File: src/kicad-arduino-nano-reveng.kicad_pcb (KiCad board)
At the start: 2 copper layers, 43.8 x 18.4 mm, 29 parts, among them J1 USB_B_Mini, J2 ISP, J3 Conn_01x15, J4 Conn_01x15, SW1 RESET, U1 AMS1117-5.0, U2 ATmega328P-AU, U3 CH340G, Y1 Crystal_Atmega, Y2 Crystal

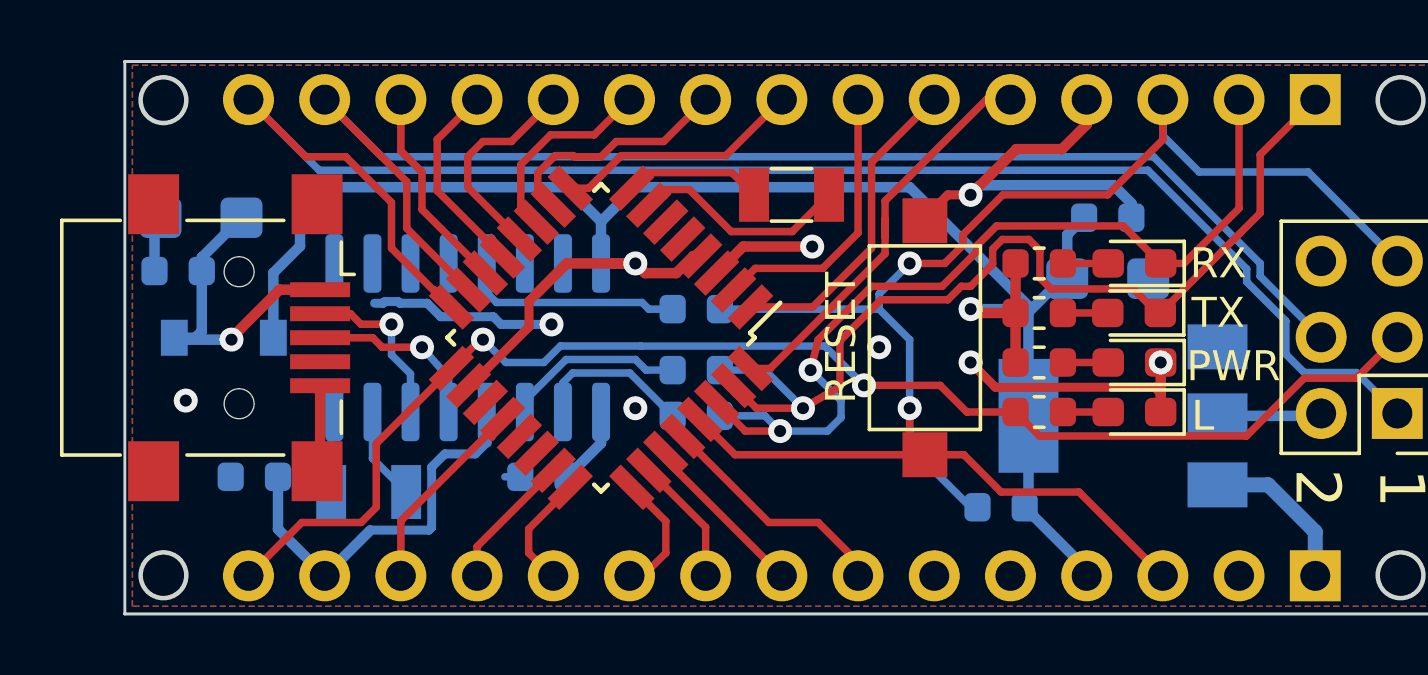
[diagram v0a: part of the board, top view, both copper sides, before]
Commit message: Finished wiring
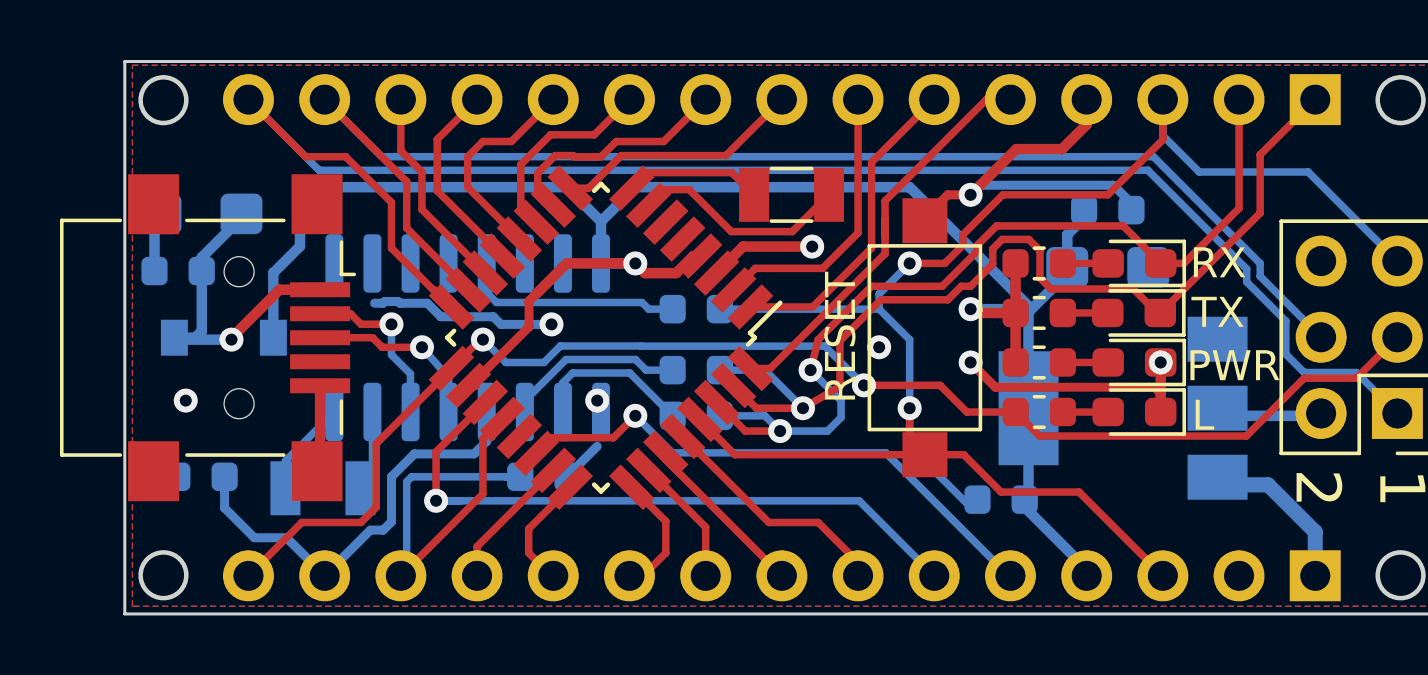
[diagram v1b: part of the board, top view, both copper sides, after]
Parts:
- U1: footprint Package_TO_SOT_SMD:SOT-223-3_TabPin2 -> igorkelvin:SOT-223-3_TabPin2
- moved C5 1.78 mm to (80.0, 61.5)
- moved Y2 1.53 mm to (84.1, 61.8)
- moved C1 0.38 mm to (110.2, 54.5)
- moved R1 0.25 mm to (106.7, 62.2)
- moved C2 0.25 mm to (110.2, 52.6)
- moved U1 0.25 mm to (110.7, 59.2)
- moved C6 0.13 mm to (80.0, 52.7)
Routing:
- net A6: track 0.00 -> 22.4 mm, vias 0 -> 1
- net A7: track 0.00 -> 18.5 mm
- net AREF: track 7.30 -> 14.4 mm
- net 3V3: track 13.4 -> 15.4 mm
- net GND: track 40.3 -> 39.3 mm, vias 7 -> 8
- net XO: track 2.71 -> 3.34 mm

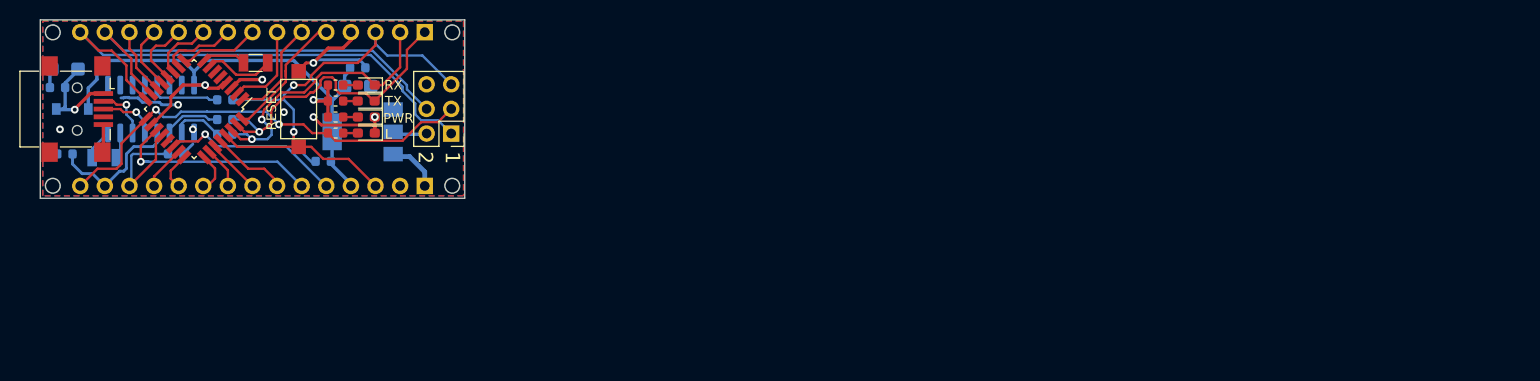
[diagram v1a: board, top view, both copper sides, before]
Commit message: PCB Rev0
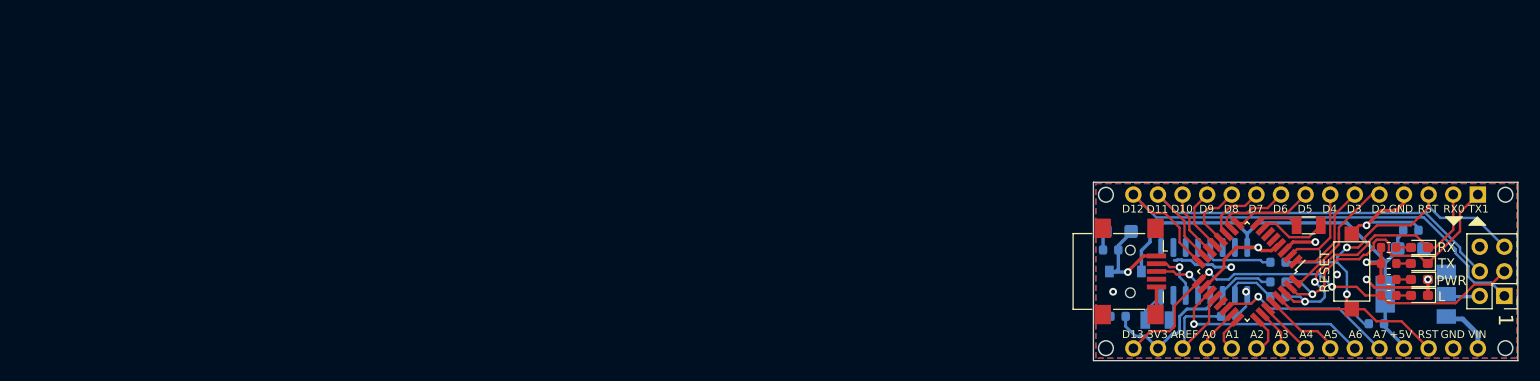
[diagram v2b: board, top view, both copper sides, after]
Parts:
- moved Y1 110.0 mm to (208.4, 68.8)
- moved C1 110.0 mm to (218.9, 71.2)
- moved C2 110.0 mm to (218.9, 69.3)
- moved C3 110.0 mm to (205.2, 72.6)
- moved C5 110.0 mm to (188.7, 78.2)
- moved C6 110.0 mm to (188.7, 69.5)
- moved C7 110.0 mm to (188.0, 71.4)
- moved D2 110.0 mm to (219.8, 72.8)
- moved D5 110.0 mm to (189.5, 73.6)
- moved R2 110.0 mm to (205.2, 74.7)
- moved R3 110.0 mm to (205.2, 76.2)
- moved R4 110.0 mm to (216.7, 71.1)
- moved R5 110.0 mm to (216.7, 72.8)
- moved R6 110.0 mm to (216.7, 74.4)
- moved R7 110.0 mm to (216.7, 76.1)
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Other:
- board text added: "+5V"
- board text added: "3V3"
- board text added: "A0"
- board text added: "A1"
- board text added: "A2"
- board text added: "A3"
- board text added: "A4"
- board text added: "A5"
- board text added: "A6"
- board text added: "A7"
- board text added: "AREF"
- board text added: "D10"
- board text added: "D11"
- board text added: "D12"
- board text added: "D13"
- board text added: "D2"
- board text added: "D3"
- board text added: "D4"
- board text added: "D5"
- board text added: "D6"
- board text added: "D7"
- board text added: "D8"
- board text added: "D9"
- board text added: "GND"
- board text added: "RST"
- board text added: "RX0"
- board text added: "TX1"
- board text added: "VIN"
- board text removed: "2"
